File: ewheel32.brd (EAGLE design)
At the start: 160 x 30.5 mm, 201 parts, among them Q1 32.768kHz, Q2 8MHz, U1 MK22DX256VLF5, U10 MC74HC595ADTR2G, U11 MC74HC595ADTR2G, U12 MC74HC595ADTR2G, U13 MC74HC595ADTR2G, U14 MC74HC595ADTR2G, U15 MC74HC595ADTR2G, U16 MC74HC595ADTR2G, U17 MC74HC595ADTR2G, U18 A3213LH, U2 MPL3115A2, U3 MMA8451QR1, U4 MCP73832T-2ACI/OT, U5 BL600, U6 MC74HC595ADTR2G, U7 MC74HC595ADTR2G, U8 MC74HC595ADTR2G, U9 MC74HC595ADTR2G, X1 PIN-HEADER-MICRO-2-5-SMD, X2 PIN-HEADER-MICRO-2-5-SMD, X4 MICRO-USB-SHIELD-ZX62R-B-5P

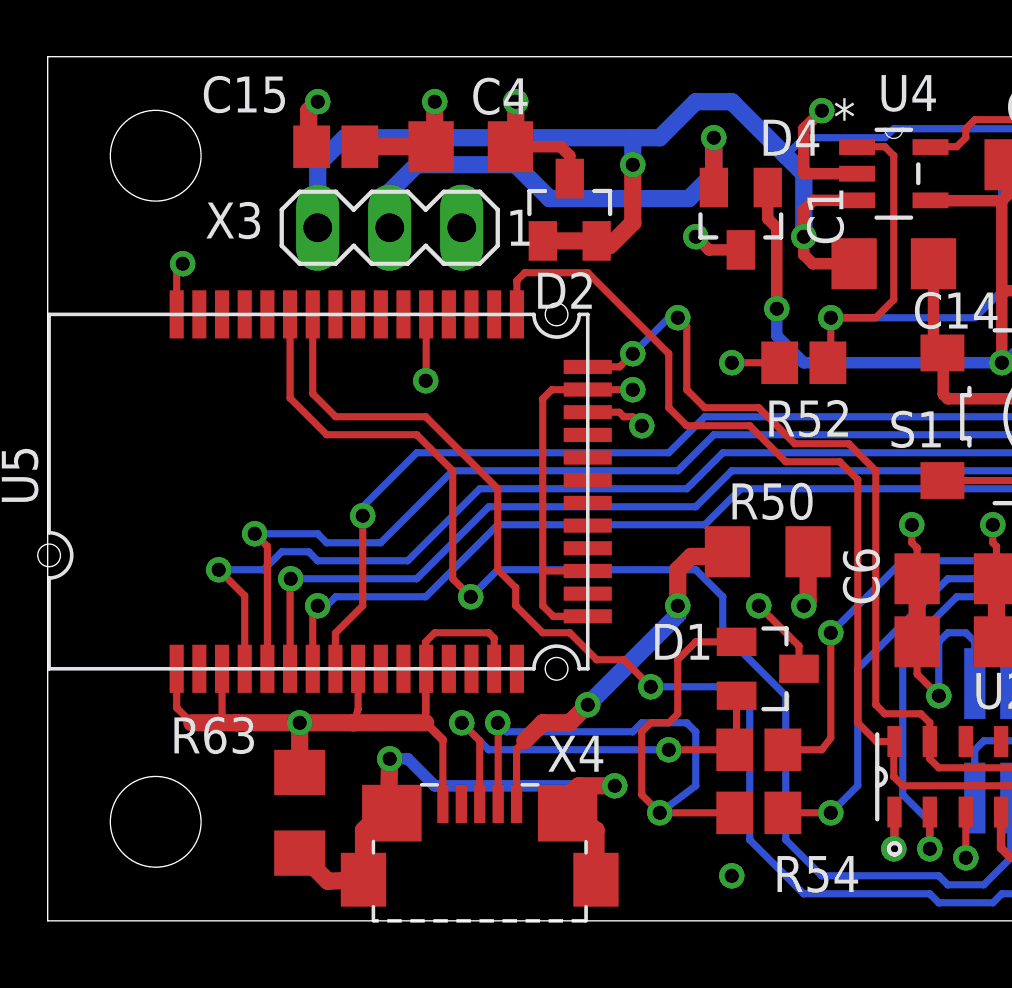
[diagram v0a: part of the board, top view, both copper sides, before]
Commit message: Intermediate version. Do not use.
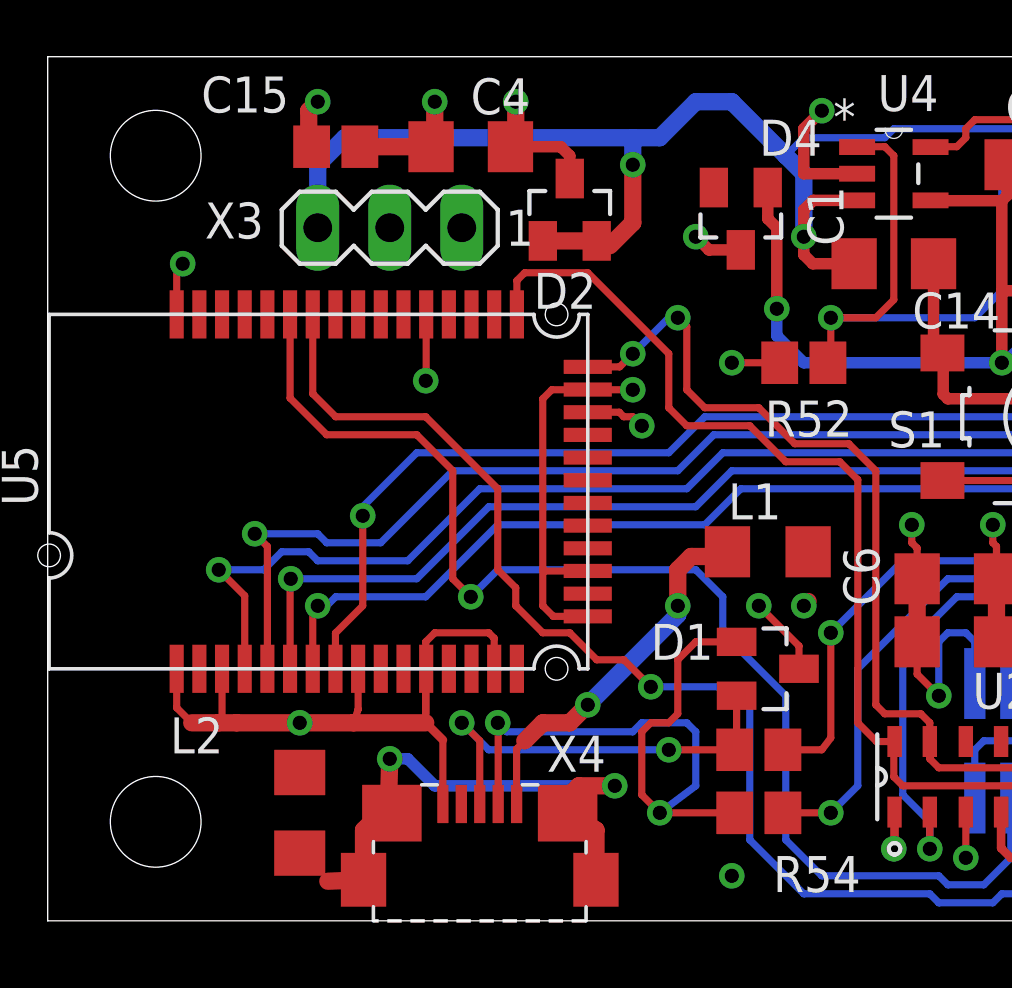
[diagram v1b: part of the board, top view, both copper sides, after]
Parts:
- removed R50, R63: 330, resistor:R1206
- added L1, L2: 3A/0.06OHM, ewheel32:L1206
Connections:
- removed net N$6: D4.2, X3.2
- new net SPI-OLED-A0: U1.40
- new net SPI-OLED-CS: U1.48
- net +5V: now also L1.2; no longer R50.2
- net GND: now also L2.2; no longer R63.1
- net N$55: now also L2.1; no longer R63.2
- net N$60: now also L1.1; no longer R50.1
- net V+: now also X3.2
- net VBAT: now also D4.2
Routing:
- net N$6: track 17.0 -> 0.00 mm, vias 1 -> 0
- net +5V: track 53.2 -> 51.4 mm
- net GND: track 202.0 -> 200.3 mm
- net N$55: track 23.4 -> 22.0 mm
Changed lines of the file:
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@@
 <attribute name="VALUE" x="38.6715" y="10.8585" size="1.27" layer="27" rot="R180"/>
 </element>
-<element name="R50" library="resistor" package="R1206" value="330" x="25.4" y="13.0175" smashed="yes">
+<element name="L1" library="ewheel32" package="L1206" value="3A/0.06OHM" x="25.4" y="13.0175" smashed="yes">
 <attribute name="NAME" x="24.003" y="14.1605" size="1.27" layer="25"/>
 <attribute name="VALUE" x="24.003" y="10.6045" size="1.27" layer="27"/>
@@
 <attribute name="VALUE" x="19.685" y="8.4328" size="1.27" layer="27" rot="R180"/>
 </element>
-<element name="R63" library="resistor" package="R1206" value="330" x="8.89" y="3.81" smashed="yes" rot="R270">
+<element name="L2" library="ewheel32" package="L1206" value="3A/0.06OHM" x="8.89" y="3.81" smashed="yes" rot="R270">
 <attribute name="NAME" x="4.318" y="5.9055" size="1.27" layer="25"/>
 <attribute name="VALUE" x="6.477" y="5.207" size="1.27" layer="27" rot="R270"/>
@@
 <contactref element="C19" pad="2"/>
 <contactref element="U5" pad="40"/>
-<contactref element="R63" pad="1"/>
 <contactref element="U1" pad="11"/>
 <contactref element="C12" pad="1"/>
@@
 <via x="32.385" y="2.2225" extent="1-16" drill="0.5" shape="octagon"/>
 <via x="24.13" y="1.5875" extent="1-16" drill="0.5" shape="octagon"/>
-<wire x1="8.89" y1="5.232" x2="8.89" y2="6.985" width="0.6096" layer="1"/>
 <via x="8.89" y="6.985" extent="1-16" drill="0.5" shape="octagon"/>
 <wire x1="10.95" y1="8.89" x2="10.95" y2="7.4575" width="0.254" layer="1"/>
@@
 <wire x1="31.56" y1="20.03" x2="31.245" y2="20.345" width="0.4064" layer="1"/>
 <wire x1="31.245" y1="20.345" x2="31.245" y2="23.1775" width="0.4064" layer="1"/>
+<contactref element="L2" pad="2"/>
+<wire x1="8.89" y1="6.985" x2="8.89" y2="2.388" width="0" layer="19" extent="1-1"/>
 </signal>
 <signal name="+3V3" class="2">
@@
 <wire x1="23.325" y1="23.665" x2="22.86" y2="24.13" width="0.4064" layer="1"/>
 <via x="22.86" y="24.13" extent="1-16" drill="0.5" shape="octagon"/>
+<contactref element="X3" pad="2"/>
 </signal>
 <signal name="UART-TX">
@@
 <contactref element="C2" pad="2"/>
 <contactref element="C14" pad="2"/>
-<contactref element="R50" pad="2"/>
 <via x="26.67" y="11.1125" extent="1-16" drill="0.5" shape="octagon"/>
 <wire x1="26.67" y1="11.1125" x2="26.67" y2="17.78" width="0.6096" layer="3"/>
 <wire x1="26.67" y1="17.78" x2="28.575" y2="19.685" width="0.6096" layer="3"/>
 <wire x1="28.575" y1="19.685" x2="33.655" y2="19.685" width="0.6096" layer="3"/>
-<wire x1="26.822" y1="13.0175" x2="26.822" y2="11.2645" width="0.6096" layer="1"/>
 <wire x1="26.822" y1="11.2645" x2="26.67" y2="11.1125" width="0.6096" layer="1"/>
 <wire x1="31.1404" y1="25.4127" x2="31.4452" y2="25.4127" width="0.4064" layer="1"/>
@@
 <wire x1="25.7175" y1="20.6375" x2="26.67" y2="19.685" width="0.4064" layer="16"/>
 <wire x1="26.67" y1="19.685" x2="33.655" y2="19.685" width="0.4064" layer="16"/>
+<contactref element="L1" pad="2"/>
+<wire x1="26.822" y1="11.2645" x2="26.822" y2="13.0175" width="0" layer="19" extent="1-1"/>
 </signal>
 <signal name="I2C-SDA">
@@
 </signal>
 <signal name="N$60">
-<contactref element="R50" pad="1"/>
 <contactref element="X4" pad="1"/>
 <wire x1="16.54" y1="4.1228" x2="16.54" y2="6.0625" width="0.254" layer="1"/>
@@
 <wire x1="22.225" y1="10.795" x2="22.225" y2="11.1125" width="0.6096" layer="16"/>
 <via x="22.225" y="11.1125" extent="1-16" drill="0.5" shape="octagon"/>
-<wire x1="23.8125" y1="12.852" x2="23.978" y2="13.0175" width="0.6096" layer="1"/>
 <wire x1="23.8125" y1="12.852" x2="22.6945" y2="12.852" width="0.6096" layer="1"/>
 <wire x1="22.6945" y1="12.852" x2="22.225" y2="12.3825" width="0.6096" layer="1"/>
 <wire x1="22.225" y1="12.3825" x2="22.225" y2="11.1125" width="0.6096" layer="1"/>
+<contactref element="L1" pad="1"/>
+<wire x1="23.8125" y1="12.852" x2="23.978" y2="13.0175" width="0" layer="19" extent="1-1"/>
 </signal>
 <signal name="N$61">
@@
 <wire x1="26.035" y1="26.9875" x2="26.67" y2="27.6225" width="0.254" layer="16"/>
 <wire x1="26.67" y1="27.6225" x2="29.5275" y2="27.6225" width="0.254" layer="16"/>
+<contactref element="D4" pad="2"/>
+<wire x1="21.59" y1="27.6225" x2="23.4975" y2="25.865" width="0" layer="19" extent="1-16"/>
 </signal>
 <signal name="BL-LINK">
@@
 <contactref element="X4" pad="M3"/>
 <contactref element="X4" pad="M2"/>
-<contactref element="R63" pad="2"/>
 <wire x1="11.14" y1="1.4478" x2="11.14" y2="3.2025" width="0.6096" layer="1"/>
 <wire x1="11.14" y1="3.2025" x2="12.065" y2="4.1275" width="0.6096" layer="1"/>
@@
 <wire x1="12.0125" y1="3.81" x2="12.14" y2="3.7978" width="0.254" layer="1"/>
 <wire x1="11.14" y1="1.4478" x2="9.881" y2="1.397" width="0.6096" layer="1"/>
-<wire x1="9.881" y1="1.397" x2="8.89" y2="2.388" width="0.6096" layer="1"/>
 <wire x1="18.415" y1="3.695" x2="18.415" y2="4.445" width="0.6096" layer="1"/>
 <wire x1="18.415" y1="4.445" x2="18.7325" y2="4.7625" width="0.6096" layer="1"/>
 <wire x1="18.7325" y1="4.7625" x2="20.0025" y2="4.7625" width="0.6096" layer="1"/>
+<contactref element="L2" pad="1"/>
+<wire x1="11.14" y1="3.2025" x2="8.89" y2="5.232" width="0" layer="19" extent="1-1"/>
 </signal>
 <signal name="N$1">
@@
 <wire x1="38.4175" y1="21.9075" x2="38.4175" y2="21.2725" width="0.254" layer="1"/>
 </signal>
-<signal name="N$6">
-<contactref element="D4" pad="2"/>
-<contactref element="X3" pad="2"/>
-<wire x1="16.51" y1="26.67" x2="17.70560625" y2="25.47439375" width="0.6096" layer="16"/>
-<wire x1="22.61689375" y1="25.47439375" x2="23.495" y2="26.3525" width="0.6096" layer="16"/>
-<wire x1="23.495" y1="26.3525" x2="23.495" y2="27.6225" width="0.6096" layer="16"/>
-<via x="23.495" y="27.6225" extent="1-16" drill="0.5" shape="octagon"/>
-<wire x1="23.495" y1="27.6225" x2="23.495" y2="25.871034375" width="0.6096" layer="1"/>
-<wire x1="23.495" y1="25.871034375" x2="23.4975" y2="25.865" width="0.6096" layer="1" curve="45"/>
-<wire x1="22.61689375" y1="25.47439375" x2="17.70560625" y2="25.47439375" width="0.6096" layer="16"/>
-<wire x1="16.51" y1="26.67" x2="13.0175" y2="26.67" width="0.6096" layer="16"/>
-<wire x1="13.0175" y1="26.67" x2="12.065" y2="25.7175" width="0.6096" layer="16"/>
-<wire x1="12.065" y1="25.7175" x2="12.065" y2="24.4475" width="0.6096" layer="16"/>
-</signal>
 <signal name="SPI-OE">
 <contactref element="U1" pad="21"/>
@@
 <wire x1="32.385" y1="27.94" x2="32.7025" y2="28.2575" width="0.254" layer="1"/>
 </signal>
+<signal name="SPI-OLED-A0">
+<contactref element="U1" pad="40"/>
+</signal>
+<signal name="SPI-OLED-CS">
+<contactref element="U1" pad="48"/>
+</signal>
 </signals>

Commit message: Version 1.4. BAT/VCC connector wrong.
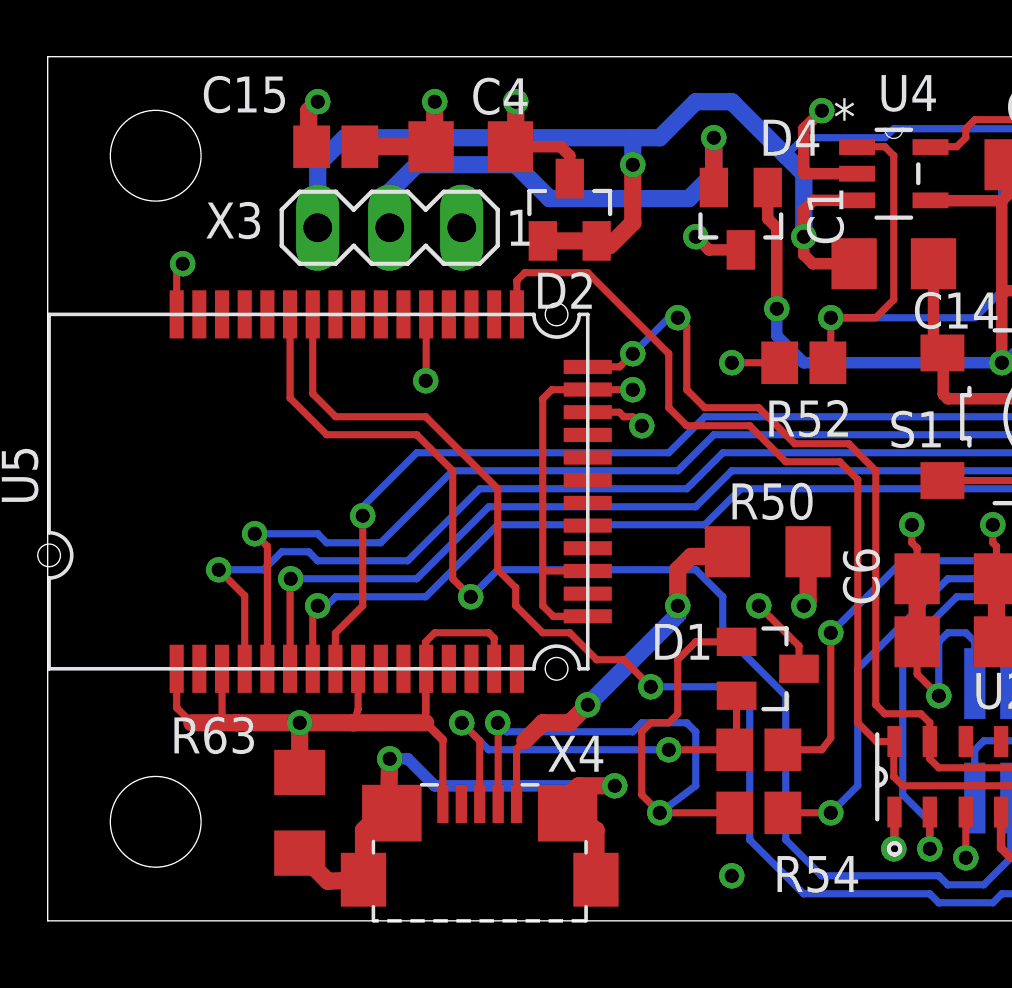
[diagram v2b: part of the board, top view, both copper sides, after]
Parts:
- removed L1, L2: 3A/0.06OHM, ewheel32:L1206
- added R50, R63: 330, resistor:R1206
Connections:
- removed net SPI-OLED-A0: U1.40
- removed net SPI-OLED-CS: U1.48
- new net N$6: D4.2, X3.2
- net +5V: now also R50.2; no longer L1.2
- net GND: now also R63.1; no longer L2.2
- net N$55: now also R63.2; no longer L2.1
- net N$60: now also R50.1; no longer L1.1
- net V+: no longer X3.2
- net VBAT: no longer D4.2
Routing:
- net N$6: track 0.00 -> 17.0 mm, vias 0 -> 1
- net +5V: track 51.4 -> 53.2 mm
- net GND: track 200.3 -> 202.0 mm
- net N$55: track 22.0 -> 23.4 mm
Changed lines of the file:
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@@
 <attribute name="VALUE" x="38.6715" y="10.8585" size="1.27" layer="27" rot="R180"/>
 </element>
-<element name="L1" library="ewheel32" package="L1206" value="3A/0.06OHM" x="25.4" y="13.0175" smashed="yes">
+<element name="R50" library="resistor" package="R1206" value="330" x="25.4" y="13.0175" smashed="yes">
 <attribute name="NAME" x="24.003" y="14.1605" size="1.27" layer="25"/>
 <attribute name="VALUE" x="24.003" y="10.6045" size="1.27" layer="27"/>
@@
 <attribute name="VALUE" x="19.685" y="8.4328" size="1.27" layer="27" rot="R180"/>
 </element>
-<element name="L2" library="ewheel32" package="L1206" value="3A/0.06OHM" x="8.89" y="3.81" smashed="yes" rot="R270">
+<element name="R63" library="resistor" package="R1206" value="330" x="8.89" y="3.81" smashed="yes" rot="R270">
 <attribute name="NAME" x="4.318" y="5.9055" size="1.27" layer="25"/>
 <attribute name="VALUE" x="6.477" y="5.207" size="1.27" layer="27" rot="R270"/>
@@
 <contactref element="C19" pad="2"/>
 <contactref element="U5" pad="40"/>
+<contactref element="R63" pad="1"/>
 <contactref element="U1" pad="11"/>
 <contactref element="C12" pad="1"/>
@@
 <via x="32.385" y="2.2225" extent="1-16" drill="0.5" shape="octagon"/>
 <via x="24.13" y="1.5875" extent="1-16" drill="0.5" shape="octagon"/>
+<wire x1="8.89" y1="5.232" x2="8.89" y2="6.985" width="0.6096" layer="1"/>
 <via x="8.89" y="6.985" extent="1-16" drill="0.5" shape="octagon"/>
 <wire x1="10.95" y1="8.89" x2="10.95" y2="7.4575" width="0.254" layer="1"/>
@@
 <wire x1="31.56" y1="20.03" x2="31.245" y2="20.345" width="0.4064" layer="1"/>
 <wire x1="31.245" y1="20.345" x2="31.245" y2="23.1775" width="0.4064" layer="1"/>
-<contactref element="L2" pad="2"/>
-<wire x1="8.89" y1="6.985" x2="8.89" y2="2.388" width="0" layer="19" extent="1-1"/>
 </signal>
 <signal name="+3V3" class="2">
@@
 <wire x1="23.325" y1="23.665" x2="22.86" y2="24.13" width="0.4064" layer="1"/>
 <via x="22.86" y="24.13" extent="1-16" drill="0.5" shape="octagon"/>
-<contactref element="X3" pad="2"/>
 </signal>
 <signal name="UART-TX">
@@
 <contactref element="C2" pad="2"/>
 <contactref element="C14" pad="2"/>
+<contactref element="R50" pad="2"/>
 <via x="26.67" y="11.1125" extent="1-16" drill="0.5" shape="octagon"/>
 <wire x1="26.67" y1="11.1125" x2="26.67" y2="17.78" width="0.6096" layer="3"/>
 <wire x1="26.67" y1="17.78" x2="28.575" y2="19.685" width="0.6096" layer="3"/>
 <wire x1="28.575" y1="19.685" x2="33.655" y2="19.685" width="0.6096" layer="3"/>
+<wire x1="26.822" y1="13.0175" x2="26.822" y2="11.2645" width="0.6096" layer="1"/>
 <wire x1="26.822" y1="11.2645" x2="26.67" y2="11.1125" width="0.6096" layer="1"/>
 <wire x1="31.1404" y1="25.4127" x2="31.4452" y2="25.4127" width="0.4064" layer="1"/>
@@
 <wire x1="25.7175" y1="20.6375" x2="26.67" y2="19.685" width="0.4064" layer="16"/>
 <wire x1="26.67" y1="19.685" x2="33.655" y2="19.685" width="0.4064" layer="16"/>
-<contactref element="L1" pad="2"/>
-<wire x1="26.822" y1="11.2645" x2="26.822" y2="13.0175" width="0" layer="19" extent="1-1"/>
 </signal>
 <signal name="I2C-SDA">
@@
 </signal>
 <signal name="N$60">
+<contactref element="R50" pad="1"/>
 <contactref element="X4" pad="1"/>
 <wire x1="16.54" y1="4.1228" x2="16.54" y2="6.0625" width="0.254" layer="1"/>
@@
 <wire x1="22.225" y1="10.795" x2="22.225" y2="11.1125" width="0.6096" layer="16"/>
 <via x="22.225" y="11.1125" extent="1-16" drill="0.5" shape="octagon"/>
+<wire x1="23.8125" y1="12.852" x2="23.978" y2="13.0175" width="0.6096" layer="1"/>
 <wire x1="23.8125" y1="12.852" x2="22.6945" y2="12.852" width="0.6096" layer="1"/>
 <wire x1="22.6945" y1="12.852" x2="22.225" y2="12.3825" width="0.6096" layer="1"/>
 <wire x1="22.225" y1="12.3825" x2="22.225" y2="11.1125" width="0.6096" layer="1"/>
-<contactref element="L1" pad="1"/>
-<wire x1="23.8125" y1="12.852" x2="23.978" y2="13.0175" width="0" layer="19" extent="1-1"/>
 </signal>
 <signal name="N$61">
@@
 <wire x1="26.035" y1="26.9875" x2="26.67" y2="27.6225" width="0.254" layer="16"/>
 <wire x1="26.67" y1="27.6225" x2="29.5275" y2="27.6225" width="0.254" layer="16"/>
-<contactref element="D4" pad="2"/>
-<wire x1="21.59" y1="27.6225" x2="23.4975" y2="25.865" width="0" layer="19" extent="1-16"/>
 </signal>
 <signal name="BL-LINK">
@@
 <contactref element="X4" pad="M3"/>
 <contactref element="X4" pad="M2"/>
+<contactref element="R63" pad="2"/>
 <wire x1="11.14" y1="1.4478" x2="11.14" y2="3.2025" width="0.6096" layer="1"/>
 <wire x1="11.14" y1="3.2025" x2="12.065" y2="4.1275" width="0.6096" layer="1"/>
@@
 <wire x1="12.0125" y1="3.81" x2="12.14" y2="3.7978" width="0.254" layer="1"/>
 <wire x1="11.14" y1="1.4478" x2="9.881" y2="1.397" width="0.6096" layer="1"/>
+<wire x1="9.881" y1="1.397" x2="8.89" y2="2.388" width="0.6096" layer="1"/>
 <wire x1="18.415" y1="3.695" x2="18.415" y2="4.445" width="0.6096" layer="1"/>
 <wire x1="18.415" y1="4.445" x2="18.7325" y2="4.7625" width="0.6096" layer="1"/>
 <wire x1="18.7325" y1="4.7625" x2="20.0025" y2="4.7625" width="0.6096" layer="1"/>
-<contactref element="L2" pad="1"/>
-<wire x1="11.14" y1="3.2025" x2="8.89" y2="5.232" width="0" layer="19" extent="1-1"/>
 </signal>
 <signal name="N$1">
@@
 <wire x1="38.4175" y1="21.9075" x2="38.4175" y2="21.2725" width="0.254" layer="1"/>
 </signal>
+<signal name="N$6">
+<contactref element="D4" pad="2"/>
+<contactref element="X3" pad="2"/>
+<wire x1="16.51" y1="26.67" x2="17.70560625" y2="25.47439375" width="0.6096" layer="16"/>
+<wire x1="22.61689375" y1="25.47439375" x2="23.495" y2="26.3525" width="0.6096" layer="16"/>
+<wire x1="23.495" y1="26.3525" x2="23.495" y2="27.6225" width="0.6096" layer="16"/>
+<via x="23.495" y="27.6225" extent="1-16" drill="0.5" shape="octagon"/>
+<wire x1="23.495" y1="27.6225" x2="23.495" y2="25.871034375" width="0.6096" layer="1"/>
+<wire x1="23.495" y1="25.871034375" x2="23.4975" y2="25.865" width="0.6096" layer="1" curve="45"/>
+<wire x1="22.61689375" y1="25.47439375" x2="17.70560625" y2="25.47439375" width="0.6096" layer="16"/>
+<wire x1="16.51" y1="26.67" x2="13.0175" y2="26.67" width="0.6096" layer="16"/>
+<wire x1="13.0175" y1="26.67" x2="12.065" y2="25.7175" width="0.6096" layer="16"/>
+<wire x1="12.065" y1="25.7175" x2="12.065" y2="24.4475" width="0.6096" layer="16"/>
+</signal>
 <signal name="SPI-OE">
 <contactref element="U1" pad="21"/>
@@
 <wire x1="32.385" y1="27.94" x2="32.7025" y2="28.2575" width="0.254" layer="1"/>
 </signal>
-<signal name="SPI-OLED-A0">
-<contactref element="U1" pad="40"/>
-</signal>
-<signal name="SPI-OLED-CS">
-<contactref element="U1" pad="48"/>
-</signal>
 </signals>
